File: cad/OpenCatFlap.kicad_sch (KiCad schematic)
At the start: 17 parts, among them P1 Outside PIR, P2 IR Barrier Outside, P3 IR Barrier Inside, P4 Servo Outside, P5 Servo Inside, P6 RFID inside, P7 RFID outside, U1 DOIT-ESP32-DEVKIT-V1, U2 AMN33111, U3 5V

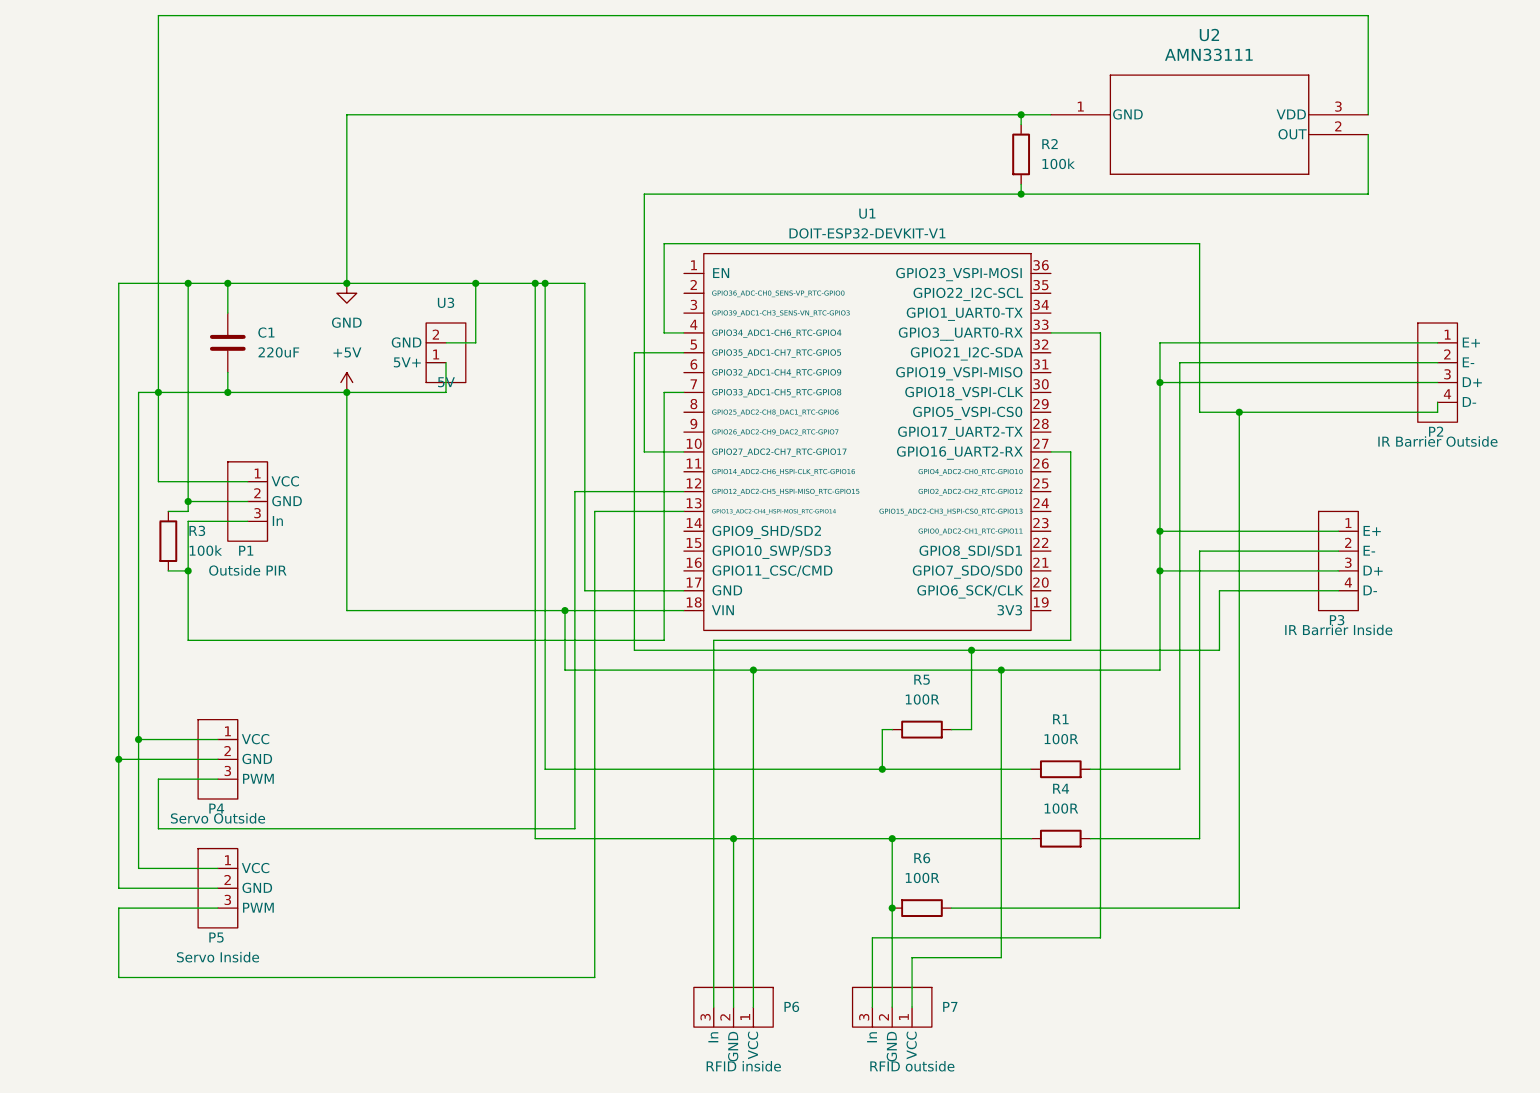
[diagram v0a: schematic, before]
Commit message: boop
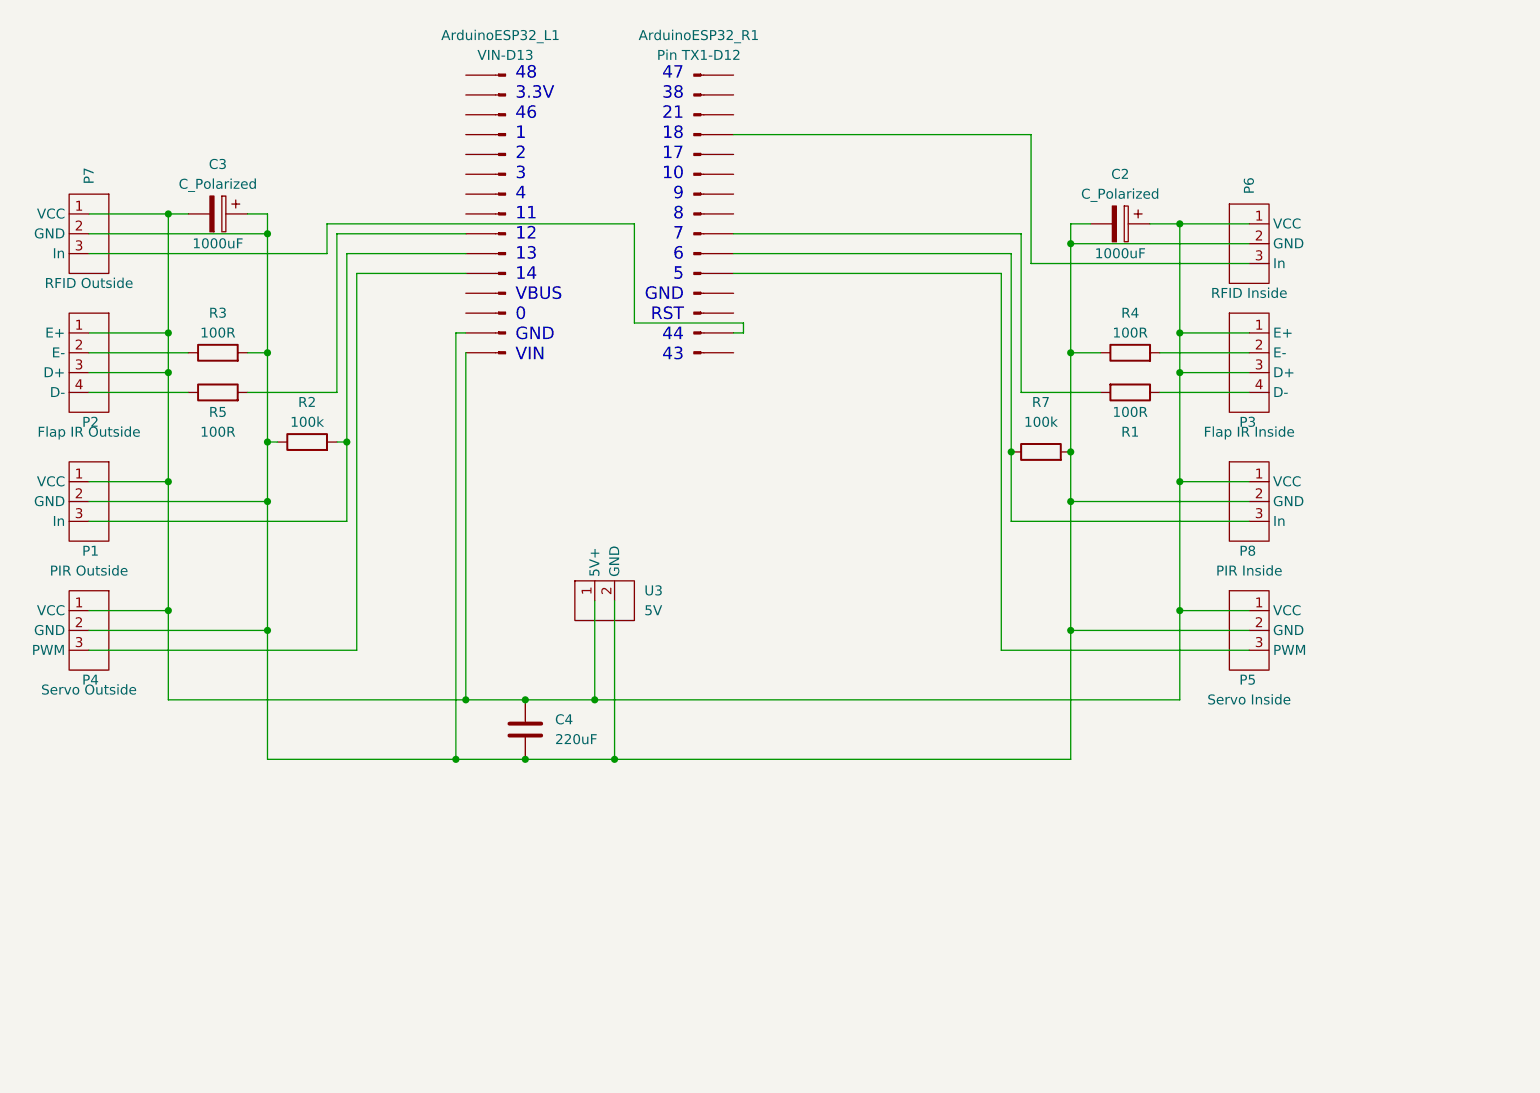
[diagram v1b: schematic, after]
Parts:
- removed C1: 220uF, Capacitor_THT:CP_Radial_D5.0mm_P2.50mm, symbol Device:C
- removed R6: 100R, Resistor_SMD:R_0805_2012Metric, symbol Device:R
- removed U1: DOIT-ESP32-DEVKIT-V1, OpenCatFlap:ESP32-DOIT-DEVKIT, symbol OpenCatFlap:DOIT-ESP32-DEVKIT-V1
- removed U2: AMN33111, OpenCatFlap:AMN33111_PAN, symbol OpenCatFlap:AMN33111
- added ArduinoESP32_L1: VIN-D13, Connector_PinHeader_2.54mm:PinHeader_1x15_P2.54mm_Vertical, symbol Connector:Conn_01x15_Pin
- added ArduinoESP32_R1: Pin TX1-D12, Connector_PinHeader_2.54mm:PinHeader_1x15_P2.54mm_Vertical, symbol Connector:Conn_01x15_Pin
- added C2, C3: C_Polarized, Capacitor_SMD:CP_Elec_8x10, symbol Device:C_Polarized
- added C4: 220uF, Capacitor_Tantalum_SMD:CP_EIA-7343-43_Kemet-X, symbol Device:C
- added P8: PIR Inside, Connector_PinHeader_2.54mm:PinHeader_1x03_P2.54mm_Vertical, symbol OpenCatFlap:PIR Header
- added R7: 100k, Resistor_SMD:R_0805_2012Metric, symbol Device:R
- P1: value Outside PIR -> PIR Outside; footprint OpenCatFlap:PIR Header -> Connector_PinHeader_2.54mm:PinHeader_1x03_P2.54mm_Vertical
- P2: value IR Barrier Outside -> Flap IR Outside; footprint OpenCatFlap:IR Barrier Header -> Connector_PinHeader_2.54mm:PinHeader_1x04_P2.54mm_Vertical
- P3: value IR Barrier Inside -> Flap IR Inside; footprint OpenCatFlap:IR Barrier Header -> Connector_PinHeader_2.54mm:PinHeader_1x04_P2.54mm_Vertical
- P4, P5: footprint OpenCatFlap:Servo Header -> Connector_PinHeader_2.54mm:PinHeader_1x03_P2.54mm_Vertical
- P6: value RFID inside -> RFID Inside; footprint OpenCatFlap:PIR Header -> Connector_PinHeader_2.54mm:PinHeader_1x03_P2.54mm_Vertical
- P7: value RFID outside -> RFID Outside; footprint OpenCatFlap:PIR Header -> Connector_PinHeader_2.54mm:PinHeader_1x03_P2.54mm_Vertical
- R3: value 100k -> 100R
- U3: footprint OpenCatFlap:Power Header -> Connector_PinHeader_2.54mm:PinHeader_1x02_P2.54mm_Vertical
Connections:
- net at P7.3 (In): now also ArduinoESP32_R1.14 (Pin_14)
- net at P2.4 (D-): now also R5.1
- net at R2.2: now also P1.3 (In), ArduinoESP32_L1.10 (Pin_10)
- net at P4.3 (PWM): now also ArduinoESP32_L1.11 (Pin_11)
- net at R3.2: now also P1.2 (GND), P4.2 (GND), P5.2 (GND), P6.2 (GND), P7.2 (GND), R2.1, R4.1, U3.2 (GND), ArduinoESP32_L1.14 (Pin_14), C2.2, C3.1, C4.2, P8.2 (GND), R7.2; no longer P1.3 (In)
- net at R1.2: now also ArduinoESP32_R1.9 (Pin_9); no longer P2.2 (E-)
- net at P5.3 (PWM): now also ArduinoESP32_R1.11 (Pin_11)
- net at P6.3 (In): now also ArduinoESP32_R1.4 (Pin_4)
- net at R5.2: now also ArduinoESP32_L1.9 (Pin_9); no longer P3.4 (D-)
- net +5V: no longer names the net of P1.1 (VCC), P2.1 (E+), P2.3 (D+), P3.1 (E+), P3.3 (D+), P4.1 (VCC), P5.1 (VCC), P6.1 (VCC), P7.1 (VCC), U3.1 (5V+)
- net +5V: now also ArduinoESP32_L1.15 (Pin_15), C2.1, C3.2, C4.1, P8.1 (VCC)
- removed net GND: P1.2 (GND), P4.2 (GND), P5.2 (GND), P6.2 (GND), P7.2 (GND), R1.1, R2.1, R3.1, R4.1, R5.1, U3.2 (GND)
- new net: ArduinoESP32_R1.10 (Pin_10), P8.3 (In), R7.1
- new net: P2.2 (E-), R3.1
- new net: P3.4 (D-), R1.1
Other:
- note added: "47 38 21 18 17 10 9 8 7 6 5 GND RST 44 43"
- note added: "48 3.3V 46 1 2 3 4 11 12 13 14 VBUS 0 GND VIN"
- moved on the sheet: P1, P2, P3, P4, P5, P6, P7, R4, U3
